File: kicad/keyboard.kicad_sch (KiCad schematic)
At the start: 84 parts, among them J1 USB_C_Receptacle_USB2.0_14P, J2 AudioJack4, J3 Conn_01x04_Pin, SW1 SW_Push, SW10 SW_Push, SW11 SW_Push, SW12 SW_Push, SW13 SW_Push, SW14 SW_Push, SW15 SW_Push, SW16 SW_Push, SW17 SW_Push, SW18 SW_Push, SW19 SW_Push, SW2 SW_Push, SW20 SW_Push, SW21 SW_Push, SW22 SW_Push, SW23 SW_Push, SW24 SW_Push, SW25 SW_Push, SW26 SW_Push, SW27 SW_Push, SW28 SW_Push, SW29 SW_Push, SW3 SW_Push, SW30 SW_Push, SW31 SW_Push, SW32 SW_Push, SW33 SW_Push, SW34 SW_Push, SW35 SW_Push, SW36 SW_Push, SW4 SW_Push, SW5 SW_Push, SW6 SW_Push, SW7 SW_Push, SW8 SW_Push, SW9 SW_Push, U1 AVR32DU32x-xPT

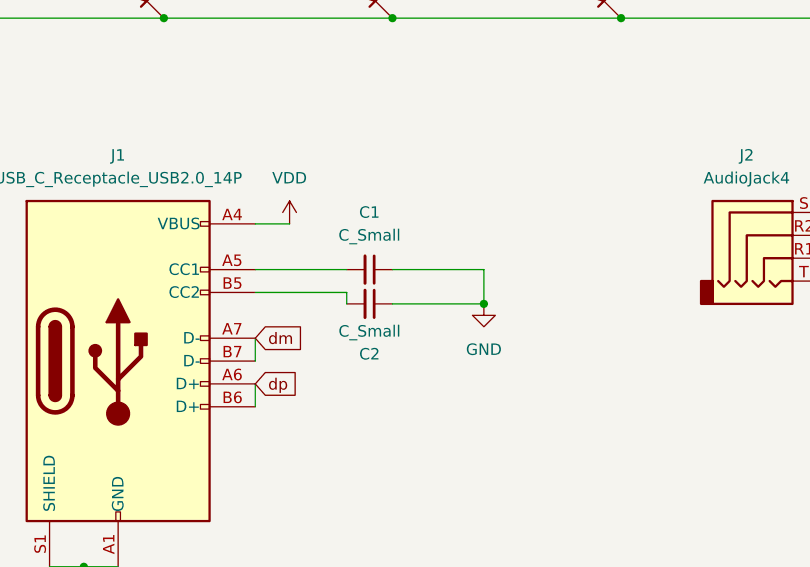
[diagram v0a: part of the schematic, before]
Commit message: saved changes to schematic
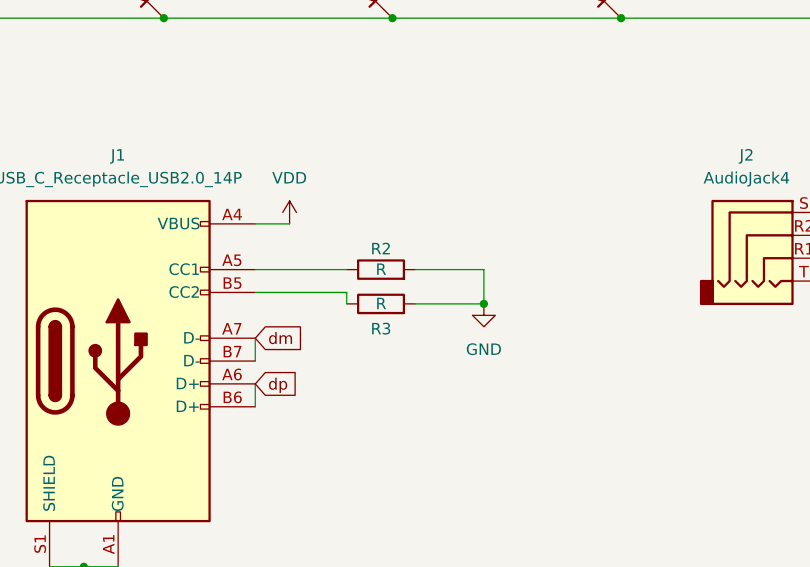
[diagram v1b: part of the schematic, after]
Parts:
- removed C1, C2: C_Small, Capacitor_THT:C_Axial_L3.8mm_D2.6mm_P7.50mm_Horizontal, symbol Device:C_Small
- added R2, R3: R, Resistor_SMD:R_0603_1608Metric, symbol Device:R
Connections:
- net GND: now also R2.2, R3.2
- net at J1.A5 (CC1): now also R2.1
- net at J1.B5 (CC2): now also R3.1
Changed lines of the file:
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@@
 	(wire
 		(pts
+			(xy 170.18 125.73) (xy 177.8 125.73)
+		)
+		(stroke
+			(width 0)
+			(type default)
+		)
+	)
+	(wire
+		(pts
 			(xy 96.52 165.1) (xy 96.52 149.86)
 		)
@@
 	(wire
 		(pts
+			(xy 170.18 121.92) (xy 177.8 121.92)
+		)
+		(stroke
+			(width 0)
+			(type default)
+		)
+	)
+	(wire
+		(pts
 			(xy 91.44 55.88) (xy 116.84 55.88)
 		)
@@
 	(wire
 		(pts
-			(xy 167.64 121.92) (xy 177.8 121.92)
-		)
-		(stroke
-			(width 0)
-			(type default)
-		)
-	)
-	(wire
-		(pts
 			(xy 66.04 172.72) (xy 67.31 172.72)
 		)
@@
 		)
 	)
-	(wire
-		(pts
-			(xy 167.64 125.73) (xy 177.8 125.73)
-		)
-		(stroke
-			(width 0)
-			(type default)
-		)
-	)
 	(global_label "col1"
 		(shape input)
@@
 	)
 	(symbol
+		(lib_id "Device:R")
+		(at 166.37 121.92 90)
+		(unit 1)
+		(exclude_from_sim no)
+		(in_bom yes)
+		(on_board yes)
+		(dnp no)
+		(property "Reference" "R2"
+			(at 166.37 119.634 90)
+			(effects
+				(font
+					(size 1.27 1.27)
+				)
+			)
+		)
+		(property "Value" "R"
+			(at 166.37 121.92 90)
+			(effects
+				(font
+					(size 1.27 1.27)
+				)
+			)
+		)
+		(property "Footprint" "Resistor_SMD:R_0603_1608Metric"
+			(at 166.37 123.698 90)
+			(effects
+				(font
+					(size 1.27 1.27)
+				)
+				(hide yes)
+			)
+		)
+		(property "Datasheet" "~"
+			(at 166.37 121.92 0)
+			(effects
+				(font
+					(size 1.27 1.27)
+				)
+				(hide yes)
+			)
+		)
+		(property "Description" "Resistor"
+			(at 166.37 121.92 0)
+			(effects
+				(font
+					(size 1.27 1.27)
+				)
+				(hide yes)
+			)
+		)
+		(pin "2"
+		)
+		(pin "1"
+		)
+		(instances
+			(project ""
+				(path "/0f30e58f-d136-47bb-bd23-5df2db91482a"
+					(reference "R2")
+					(unit 1)
+				)
+			)
+		)
+	)
+	(symbol
 		(lib_id "power:GND")
 		(at 102.87 142.24 90)
@@
 	)
 	(symbol
+		(lib_id "Device:R")
+		(at 166.37 125.73 90)
+		(unit 1)
+		(exclude_from_sim no)
+		(in_bom yes)
+		(on_board yes)
+		(dnp no)
+		(property "Reference" "R3"
+			(at 166.37 128.524 90)
+			(effects
+				(font
+					(size 1.27 1.27)
+				)
+			)
+		)
+		(property "Value" "R"
+			(at 166.37 125.73 90)
+			(effects
+				(font
+					(size 1.27 1.27)
+				)
+			)
+		)
+		(property "Footprint" "Resistor_SMD:R_0603_1608Metric"
+			(at 166.37 127.508 90)
+			(effects
+				(font
+					(size 1.27 1.27)
+				)
+				(hide yes)
+			)
+		)
+		(property "Datasheet" "~"
+			(at 166.37 125.73 0)
+			(effects
+				(font
+					(size 1.27 1.27)
+				)
+				(hide yes)
+			)
+		)
+		(property "Description" "Resistor"
+			(at 166.37 125.73 0)
+			(effects
+				(font
+					(size 1.27 1.27)
+				)
+				(hide yes)
+			)
+		)
+		(pin "2"
+		)
+		(pin "1"
+		)
+		(instances
+			(project "keyboard"
+				(path "/0f30e58f-d136-47bb-bd23-5df2db91482a"
+					(reference "R3")
+					(unit 1)
+				)
+			)
+		)
+	)
+	(symbol
 		(lib_id "Switch:SW_Push")
 		(at 157.48 88.9 0)
@@
 	)
 	(symbol
-		(lib_id "Device:C_Small")
-		(at 165.1 125.73 270)
-		(unit 1)
-		(exclude_from_sim no)
-		(in_bom yes)
-		(on_board yes)
-		(dnp no)
-		(property "Reference" "C2"
-			(at 165.1 131.318 90)
-			(effects
-				(font
-					(size 1.27 1.27)
-				)
-			)
-		)
-		(property "Value" "C_Small"
-			(at 165.1 128.778 90)
-			(effects
-				(font
-					(size 1.27 1.27)
-				)
-			)
-		)
-		(property "Footprint" "Capacitor_THT:C_Axial_L3.8mm_D2.6mm_P7.50mm_Horizontal"
-			(at 165.1 125.73 0)
-			(effects
-				(font
-					(size 1.27 1.27)
-				)
-				(hide yes)
-			)
-		)
-		(property "Datasheet" "~"
-			(at 165.1 125.73 0)
-			(effects
-				(font
-					(size 1.27 1.27)
-				)
-				(hide yes)
-			)
-		)
-		(property "Description" "Unpolarized capacitor, small symbol"
-			(at 165.1 125.73 0)
-			(effects
-				(font
-					(size 1.27 1.27)
-				)
-				(hide yes)
-			)
-		)
-		(pin "2"
-		)
-		(pin "1"
-		)
-		(instances
-			(project "kicad"
-				(path "/0f30e58f-d136-47bb-bd23-5df2db91482a"
-					(reference "C2")
-					(unit 1)
-				)
-			)
-		)
-	)
-	(symbol
 		(lib_id "Switch:SW_Push")
 		(at 81.28 38.1 0)
@@
 					(unit 1)
 				)
-			)
-		)
-	)
-	(symbol
-		(lib_id "Device:C_Small")
-		(at 165.1 121.92 270)
-		(unit 1)
-		(exclude_from_sim no)
-		(in_bom yes)
-		(on_board yes)
-		(dnp no)
-		(fields_autoplaced yes)
-		(property "Reference" "C1"
-			(at 165.0936 115.57 90)
-			(effects
-				(font
-					(size 1.27 1.27)
-				)
-			)
-		)
-		(property "Value" "C_Small"
-			(at 165.0936 118.11 90)
-			(effects
-				(font
-					(size 1.27 1.27)
-				)
-			)
-		)
-		(property "Footprint" "Capacitor_THT:C_Axial_L3.8mm_D2.6mm_P7.50mm_Horizontal"
-			(at 165.1 121.92 0)
-			(effects
-				(font
-					(size 1.27 1.27)
-				)
-				(hide yes)
-			)
-		)
-		(property "Datasheet" "~"
-			(at 165.1 121.92 0)
-			(effects
-				(font
-					(size 1.27 1.27)
-				)
-				(hide yes)
-			)
-		)
-		(property "Description" "Unpolarized capacitor, small symbol"
-			(at 165.1 121.92 0)
-			(effects
-				(font
-					(size 1.27 1.27)
-				)
-				(hide yes)
-			)
-		)
-		(pin "2"
-		)
-		(pin "1"
-		)
-		(instances
-			(project ""
-				(path "/0f30e58f-d136-47bb-bd23-5df2db91482a"
-					(reference "C1")
-					(unit 1)
-				)

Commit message: finished up left-side pcb, not sure if right should go in the same project or to make a new one, plotted gerber files
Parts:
- C3, C4, C5, C6, C7: footprint Capacitor_THT:C_Axial_L3.8mm_D2.6mm_P7.50mm_Horizontal -> Capacitor_SMD:C_0603_1608Metric
- D1, D10, D11, D12, D13, D14, D15, D16, D17, D18, D19, D2, D20, D21, D22, D23, D24, D25, D26, D27, D28, D29, D3, D30, D31, D32, D33, D34, D35, D4, D5, D6, D7, D8, D9: footprint Diode_SMD:D_SMB -> Diode_THT:D_DO-35_SOD27_P3.81mm_Vertical_AnodeUp
- RV1: footprint Potentiometer_THT:Potentiometer_ACP_CA9-V10_Vertical_Hole -> Potentiometer_THT:Potentiometer_TT_P0915N
- SW1, SW2, SW3, SW34, SW4, SW5: footprint Button_Switch_Keyboard:SW_Cherry_MX_1.00u_PCB -> Button_Switch_Keyboard:SW_Cherry_MX_1.50u_PCB
- SW33: footprint Button_Switch_Keyboard:SW_Cherry_MX_1.00u_PCB -> Button_Switch_Keyboard:SW_Cherry_MX_1.25u_PCB
- SW35: footprint Button_Switch_Keyboard:SW_Cherry_MX_1.00u_PCB -> Button_Switch_Keyboard:SW_Cherry_MX_1.75u_PCB
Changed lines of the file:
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@@
 			)
 		)
-		(property "Footprint" "Diode_SMD:D_SMB"
+		(property "Footprint" "Diode_THT:D_DO-35_SOD27_P3.81mm_Vertical_AnodeUp"
 			(at 165.1 78.74 0)
 			(effects
@@
 			)
 		)
-		(property "Footprint" "Diode_SMD:D_SMB"
+		(property "Footprint" "Diode_THT:D_DO-35_SOD27_P3.81mm_Vertical_AnodeUp"
 			(at 88.9 53.34 0)
 			(effects
@@
 			)
 		)
-		(property "Footprint" "Diode_SMD:D_SMB"
+		(property "Footprint" "Diode_THT:D_DO-35_SOD27_P3.81mm_Vertical_AnodeUp"
 			(at 63.5 53.34 0)
 			(effects
@@
 			)
 		)
-		(property "Footprint" "Diode_SMD:D_SMB"
+		(property "Footprint" "Diode_THT:D_DO-35_SOD27_P3.81mm_Vertical_AnodeUp"
 			(at 165.1 40.64 0)
 			(effects
@@
 			)
 		)
-		(property "Footprint" "Diode_SMD:D_SMB"
+		(property "Footprint" "Diode_THT:D_DO-35_SOD27_P3.81mm_Vertical_AnodeUp"
 			(at 190.5 78.74 0)
 			(effects
@@
 			)
 		)
-		(property "Footprint" "Button_Switch_Keyboard:SW_Cherry_MX_1.00u_PCB"
+		(property "Footprint" "Button_Switch_Keyboard:SW_Cherry_MX_1.75u_PCB"
 			(at 208.28 83.82 0)
 			(effects
@@
 			)
 		)
-		(property "Footprint" "Diode_SMD:D_SMB"
+		(property "Footprint" "Diode_THT:D_DO-35_SOD27_P3.81mm_Vertical_AnodeUp"
 			(at 190.5 91.44 0)
 			(effects
@@
 			)
 		)
-		(property "Footprint" "Button_Switch_Keyboard:SW_Cherry_MX_1.00u_PCB"
+		(property "Footprint" "Button_Switch_Keyboard:SW_Cherry_MX_1.50u_PCB"
 			(at 208.28 71.12 0)
 			(effects
@@
 			)
 		)
-		(property "Footprint" "Diode_SMD:D_SMB"
+		(property "Footprint" "Diode_THT:D_DO-35_SOD27_P3.81mm_Vertical_AnodeUp"
 			(at 139.7 53.34 0)
 			(effects
@@
 			)
 		)
-		(property "Footprint" "Capacitor_THT:C_Axial_L3.8mm_D2.6mm_P7.50mm_Horizontal"
+		(property "Footprint" "Capacitor_SMD:C_0603_1608Metric"
 			(at 33.02 154.94 0)
 			(effects
@@
 			)
 		)
-		(property "Footprint" "Diode_SMD:D_SMB"
+		(property "Footprint" "Diode_THT:D_DO-35_SOD27_P3.81mm_Vertical_AnodeUp"
 			(at 63.5 40.64 0)
 			(effects
@@
 			)
 		)
-		(property "Footprint" "Diode_SMD:D_SMB"
+		(property "Footprint" "Diode_THT:D_DO-35_SOD27_P3.81mm_Vertical_AnodeUp"
 			(at 190.5 53.34 0)
 			(effects
@@
 			)
 		)
-		(property "Footprint" "Diode_SMD:D_SMB"
+		(property "Footprint" "Diode_THT:D_DO-35_SOD27_P3.81mm_Vertical_AnodeUp"
 			(at 63.5 78.74 0)
 			(effects
@@
 			)
 		)
-		(property "Footprint" "Button_Switch_Keyboard:SW_Cherry_MX_1.00u_PCB"
+		(property "Footprint" "Button_Switch_Keyboard:SW_Cherry_MX_1.50u_PCB"
 			(at 55.88 83.82 0)
 			(effects
@@
 			)
 		)
-		(property "Footprint" "Diode_SMD:D_SMB"
+		(property "Footprint" "Diode_THT:D_DO-35_SOD27_P3.81mm_Vertical_AnodeUp"
 			(at 215.9 40.64 0)
 			(effects
@@
 			)
 		)
-		(property "Footprint" "Diode_SMD:D_SMB"
+		(property "Footprint" "Diode_THT:D_DO-35_SOD27_P3.81mm_Vertical_AnodeUp"
 			(at 165.1 66.04 0)
 			(effects
@@
 			)
 		)
-		(property "Footprint" "Diode_SMD:D_SMB"
+		(property "Footprint" "Diode_THT:D_DO-35_SOD27_P3.81mm_Vertical_AnodeUp"
 			(at 139.7 66.04 0)
 			(effects
@@
 			)
 		)
-		(property "Footprint" "Diode_SMD:D_SMB"
+		(property "Footprint" "Diode_THT:D_DO-35_SOD27_P3.81mm_Vertical_AnodeUp"
 			(at 114.3 78.74 0)
 			(effects
@@
 			)
 		)
-		(property "Footprint" "Button_Switch_Keyboard:SW_Cherry_MX_1.00u_PCB"
+		(property "Footprint" "Button_Switch_Keyboard:SW_Cherry_MX_1.50u_PCB"
 			(at 55.88 71.12 0)
 			(effects
@@
 			)
 		)
-		(property "Footprint" "Diode_SMD:D_SMB"
+		(property "Footprint" "Diode_THT:D_DO-35_SOD27_P3.81mm_Vertical_AnodeUp"
 			(at 88.9 40.64 0)
 			(effects
@@
 			)
 		)
-		(property "Footprint" "Diode_SMD:D_SMB"
+		(property "Footprint" "Diode_THT:D_DO-35_SOD27_P3.81mm_Vertical_AnodeUp"
 			(at 63.5 91.44 0)
 			(effects
@@
 			)
 		)
-		(property "Footprint" "Diode_SMD:D_SMB"
+		(property "Footprint" "Diode_THT:D_DO-35_SOD27_P3.81mm_Vertical_AnodeUp"
 			(at 165.1 53.34 0)
 			(effects
@@
 			)
 		)
-		(property "Footprint" "Capacitor_THT:C_Axial_L3.8mm_D2.6mm_P7.50mm_Horizontal"
+		(property "Footprint" "Capacitor_SMD:C_0603_1608Metric"
 			(at 74.93 111.76 0)
 			(effects
@@
 			)
 		)
-		(property "Footprint" "Diode_SMD:D_SMB"
+		(property "Footprint" "Diode_THT:D_DO-35_SOD27_P3.81mm_Vertical_AnodeUp"
 			(at 165.1 91.44 0)
 			(effects
@@
 			)
 		)
-		(property "Footprint" "Button_Switch_Keyboard:SW_Cherry_MX_1.00u_PCB"
+		(property "Footprint" "Button_Switch_Keyboard:SW_Cherry_MX_1.50u_PCB"
 			(at 55.88 33.02 0)
 			(effects
@@
 			)
 		)
-		(property "Footprint" "Button_Switch_Keyboard:SW_Cherry_MX_1.00u_PCB"
+		(property "Footprint" "Button_Switch_Keyboard:SW_Cherry_MX_1.50u_PCB"
 			(at 55.88 58.42 0)
 			(effects
@@
 			)
 		)
-		(property "Footprint" "Diode_SMD:D_SMB"
+		(property "Footprint" "Diode_THT:D_DO-35_SOD27_P3.81mm_Vertical_AnodeUp"
 			(at 114.3 91.44 0)
 			(effects
@@
 			)
 		)
-		(property "Footprint" "Diode_SMD:D_SMB"
+		(property "Footprint" "Diode_THT:D_DO-35_SOD27_P3.81mm_Vertical_AnodeUp"
 			(at 139.7 91.44 0)
 			(effects
@@
 			)
 		)
-		(property "Footprint" "Diode_SMD:D_SMB"
+		(property "Footprint" "Diode_THT:D_DO-35_SOD27_P3.81mm_Vertical_AnodeUp"
 			(at 139.7 78.74 0)
 			(effects
@@
 			)
 		)
-		(property "Footprint" "Diode_SMD:D_SMB"
+		(property "Footprint" "Diode_THT:D_DO-35_SOD27_P3.81mm_Vertical_AnodeUp"
 			(at 215.9 78.74 0)
 			(effects
@@
 			)
 		)
-		(property "Footprint" "Diode_SMD:D_SMB"
+		(property "Footprint" "Diode_THT:D_DO-35_SOD27_P3.81mm_Vertical_AnodeUp"
 			(at 139.7 40.64 0)
 			(effects
@@
 			)
 		)
-		(property "Footprint" "Diode_SMD:D_SMB"
+		(property "Footprint" "Diode_THT:D_DO-35_SOD27_P3.81mm_Vertical_AnodeUp"
 			(at 88.9 66.04 0)
 			(effects
@@
 			)
 		)
-		(property "Footprint" "Diode_SMD:D_SMB"
+		(property "Footprint" "Diode_THT:D_DO-35_SOD27_P3.81mm_Vertical_AnodeUp"
 			(at 215.9 66.04 0)
 			(effects
@@
 			)
 		)
-		(property "Footprint" "Diode_SMD:D_SMB"
+		(property "Footprint" "Diode_THT:D_DO-35_SOD27_P3.81mm_Vertical_AnodeUp"
 			(at 88.9 91.44 0)
 			(effects
@@
 			)
 		)
-		(property "Footprint" "Capacitor_THT:C_Axial_L3.8mm_D2.6mm_P7.50mm_Horizontal"
+		(property "Footprint" "Capacitor_SMD:C_0603_1608Metric"
 			(at 34.29 130.81 0)
 			(effects
@@
 			)
 		)
-		(property "Footprint" "Diode_SMD:D_SMB"
+		(property "Footprint" "Diode_THT:D_DO-35_SOD27_P3.81mm_Vertical_AnodeUp"
 			(at 114.3 66.04 0)
 			(effects
@@
 			)
 		)
-		(property "Footprint" "Diode_SMD:D_SMB"
+		(property "Footprint" "Diode_THT:D_DO-35_SOD27_P3.81mm_Vertical_AnodeUp"
 			(at 63.5 66.04 0)
 			(effects
@@
 			)
 		)
-		(property "Footprint" "Button_Switch_Keyboard:SW_Cherry_MX_1.00u_PCB"
+		(property "Footprint" "Button_Switch_Keyboard:SW_Cherry_MX_1.50u_PCB"
 			(at 55.88 45.72 0)
 			(effects
@@
 			)
 		)
-		(property "Footprint" "Capacitor_THT:C_Axial_L3.8mm_D2.6mm_P7.50mm_Horizontal"
+		(property "Footprint" "Capacitor_SMD:C_0603_1608Metric"
 			(at 59.69 111.76 0)
 			(effects
@@
 			)
 		)
-		(property "Footprint" "Diode_SMD:D_SMB"
+		(property "Footprint" "Diode_THT:D_DO-35_SOD27_P3.81mm_Vertical_AnodeUp"
 			(at 88.9 78.74 0)
 			(effects
@@
 			)
 		)
-		(property "Footprint" "Capacitor_THT:C_Axial_L3.8mm_D2.6mm_P7.50mm_Horizontal"
+		(property "Footprint" "Capacitor_SMD:C_0603_1608Metric"
 			(at 100.33 142.24 0)
 			(effects
@@
 			)
 		)
-		(property "Footprint" "Button_Switch_Keyboard:SW_Cherry_MX_1.00u_PCB"
+		(property "Footprint" "Button_Switch_Keyboard:SW_Cherry_MX_1.25u_PCB"
 			(at 208.28 58.42 0)
 			(effects
@@
 			)
 		)
-		(property "Footprint" "Diode_SMD:D_SMB"
+		(property "Footprint" "Diode_THT:D_DO-35_SOD27_P3.81mm_Vertical_AnodeUp"
 			(at 114.3 40.64 0)
 			(effects
@@
 			)
 		)
-		(property "Footprint" "Potentiometer_THT:Potentiometer_ACP_CA9-V10_Vertical_Hole"
+		(property "Footprint" "Potentiometer_THT:Potentiometer_TT_P0915N"
 			(at 101.6 165.1 0)
 			(effects
@@
 			)
 		)
-		(property "Footprint" "Diode_SMD:D_SMB"
+		(property "Footprint" "Diode_THT:D_DO-35_SOD27_P3.81mm_Vertical_AnodeUp"
 			(at 215.9 53.34 0)
 			(effects
@@
 			)
 		)
-		(property "Footprint" "Diode_SMD:D_SMB"
+		(property "Footprint" "Diode_THT:D_DO-35_SOD27_P3.81mm_Vertical_AnodeUp"
 			(at 114.3 53.34 0)
 			(effects
@@
 			)
 		)
-		(property "Footprint" "Diode_SMD:D_SMB"
+		(property "Footprint" "Diode_THT:D_DO-35_SOD27_P3.81mm_Vertical_AnodeUp"
 			(at 190.5 40.64 0)
 			(effects
@@
 			)
 		)
-		(property "Footprint" "Diode_SMD:D_SMB"
+		(property "Footprint" "Diode_THT:D_DO-35_SOD27_P3.81mm_Vertical_AnodeUp"
 			(at 190.5 66.04 0)
 			(effects
@@
 			)
 		)
-		(property "Footprint" "Diode_SMD:D_SMB"
+		(property "Footprint" "Diode_THT:D_DO-35_SOD27_P3.81mm_Vertical_AnodeUp"
 			(at 215.9 91.44 0)
 			(effects
